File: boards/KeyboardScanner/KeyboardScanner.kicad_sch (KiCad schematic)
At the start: 20 parts, among them J1 Keyboard1, J2 Keyboard1, J3 Encoder, J4 Select, U5 ULN2803A, U8 4069

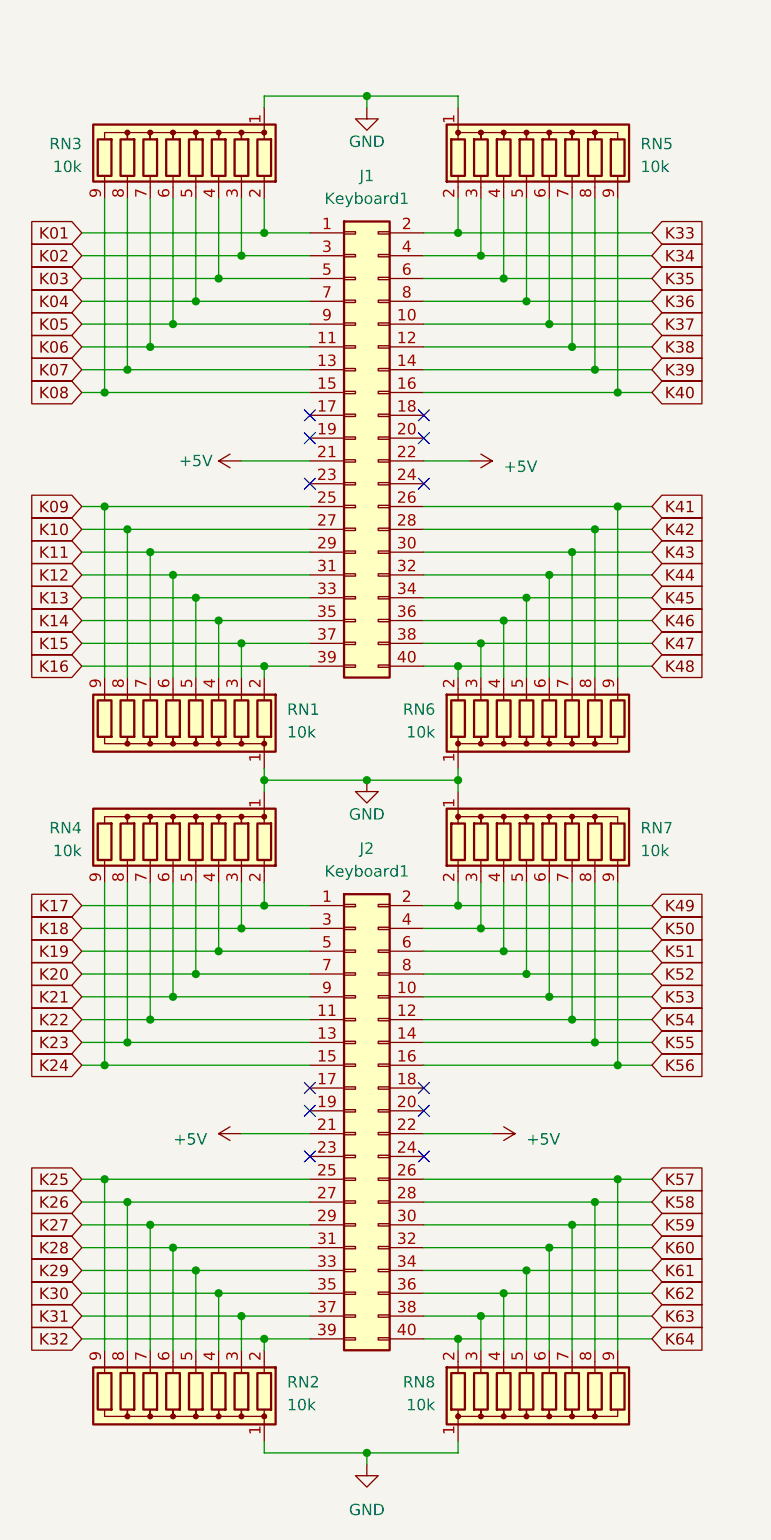
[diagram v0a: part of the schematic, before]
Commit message: Fixed KeyboardScanner schematics to fix open collector enable output
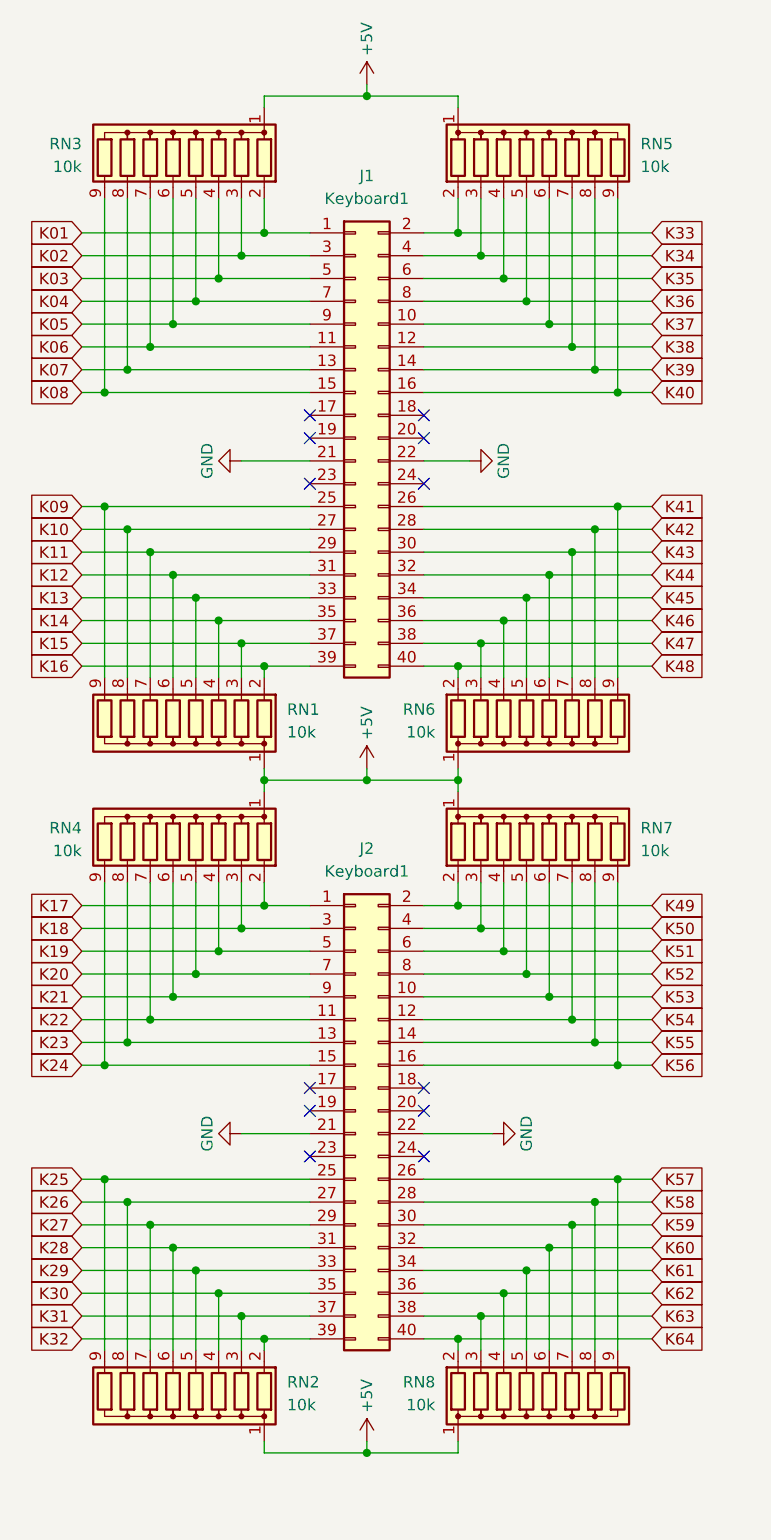
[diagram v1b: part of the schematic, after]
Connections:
- net +5V: now also RN1.1 (common), RN2.1 (common), RN3.1 (common), RN4.1 (common), RN5.1 (common), RN6.1 (common), RN7.1 (common), RN8.1 (common); no longer J1.21 (Pin_21), J1.22 (Pin_22), J2.21 (Pin_21), J2.22 (Pin_22)
- net GND: now also J1.21 (Pin_21), J1.22 (Pin_22), J2.21 (Pin_21), J2.22 (Pin_22); no longer RN1.1 (common), RN2.1 (common), RN3.1 (common), RN4.1 (common), RN5.1 (common), RN6.1 (common), RN7.1 (common), RN8.1 (common)

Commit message: Revert "Fixed KeyboardScanner schematics to fix open collector enable output"
This reverts commit 57decbb2314c6d76a4ad6cd92ca682e4977913ef.
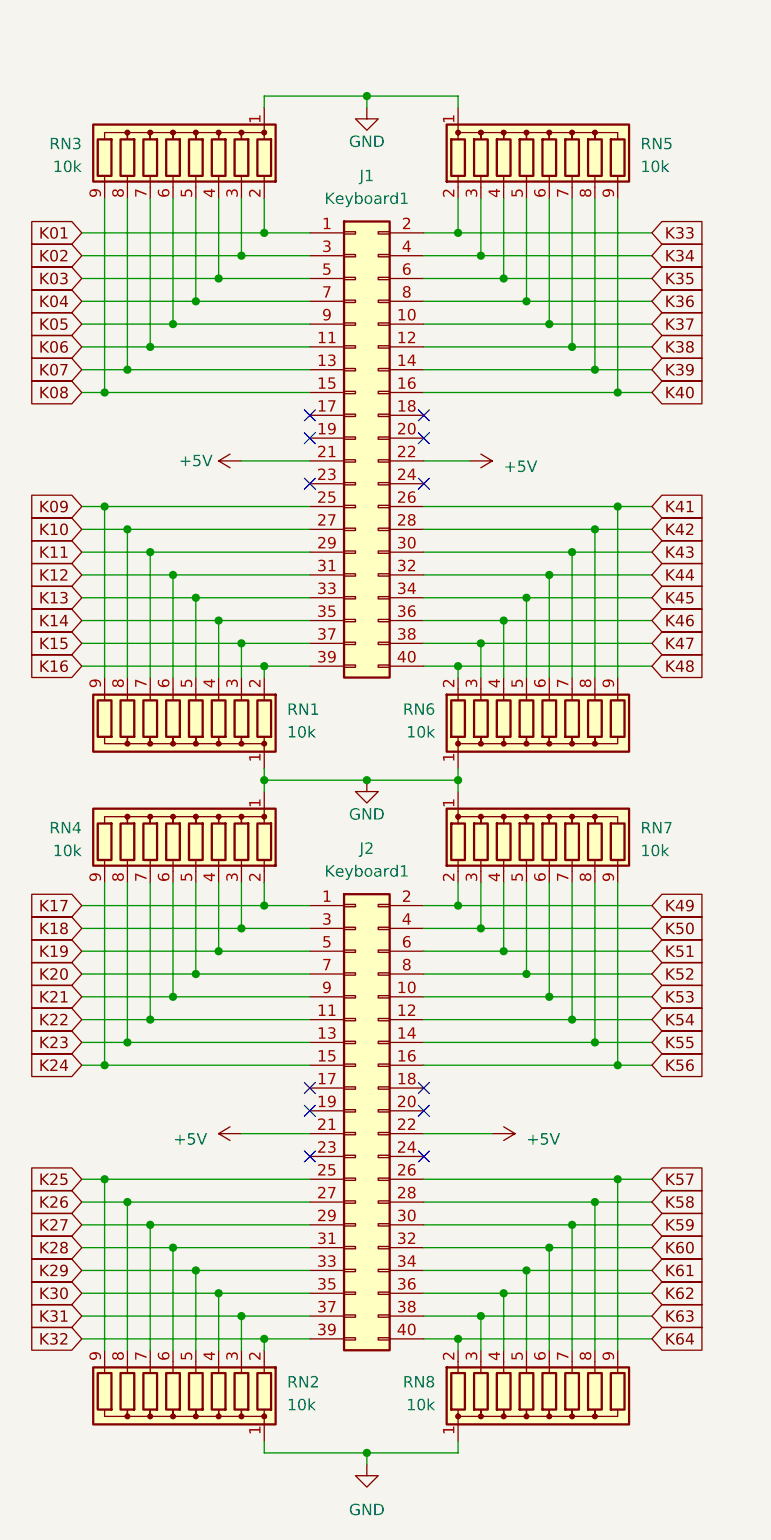
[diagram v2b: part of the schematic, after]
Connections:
- net +5V: now also J1.21 (Pin_21), J1.22 (Pin_22), J2.21 (Pin_21), J2.22 (Pin_22); no longer RN1.1 (common), RN2.1 (common), RN3.1 (common), RN4.1 (common), RN5.1 (common), RN6.1 (common), RN7.1 (common), RN8.1 (common)
- net GND: now also RN1.1 (common), RN2.1 (common), RN3.1 (common), RN4.1 (common), RN5.1 (common), RN6.1 (common), RN7.1 (common), RN8.1 (common); no longer J1.21 (Pin_21), J1.22 (Pin_22), J2.21 (Pin_21), J2.22 (Pin_22)

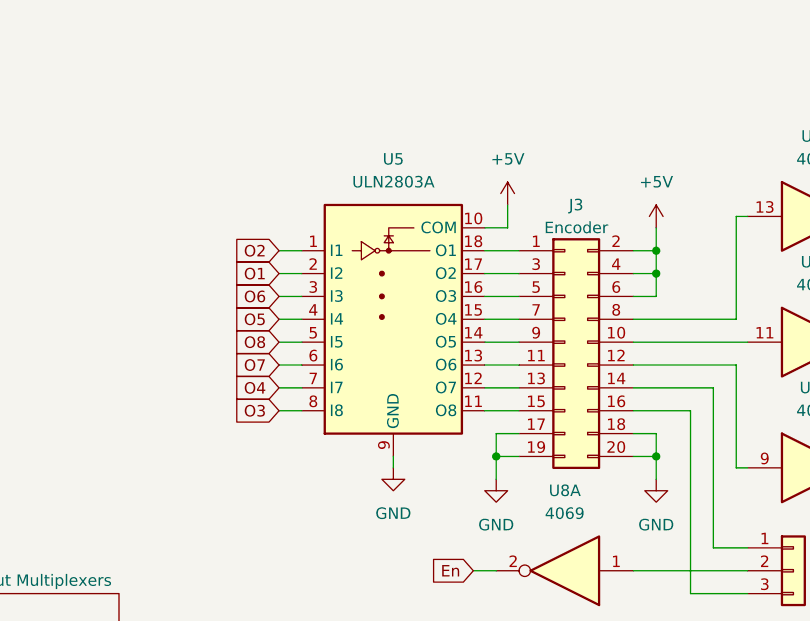
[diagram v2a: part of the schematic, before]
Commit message: Replaced inverting with non-inverting output buffer in KeyboardScanner to fix disabled open collector output
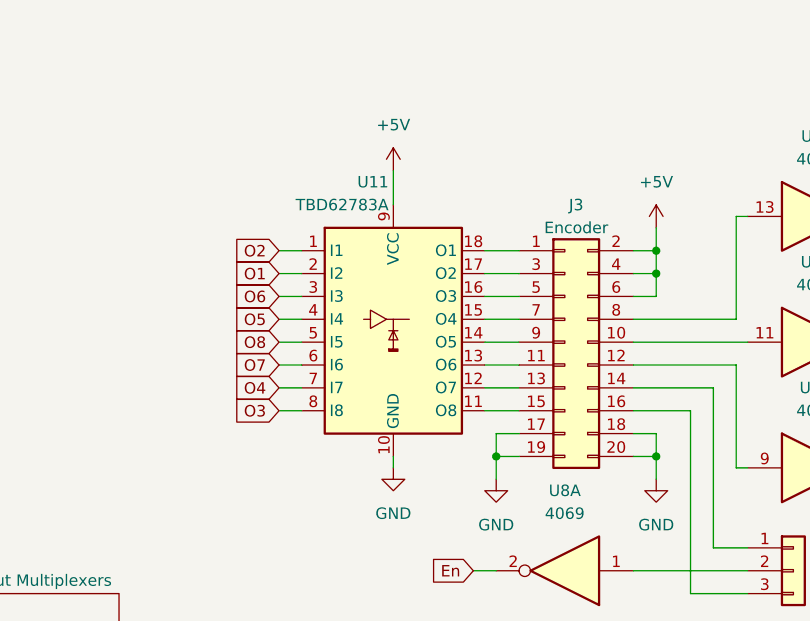
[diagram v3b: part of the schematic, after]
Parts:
- removed U5: ULN2803A, Package_DIP:DIP-18_W7.62mm, symbol Transistor_Array:ULN2803A
- added U11: TBD62783A, Package_DIP:DIP-18_W7.62mm, symbol Transistor_Array:TBD62783A
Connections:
- net +5V: now also U11.9 (VCC)
- net GND: now also U11.10 (GND)
- net O1: now also U11.2 (I2)
- net O2: now also U11.1 (I1)
- net O3: now also U11.8 (I8)
- net O4: now also U11.7 (I7)
- net O5: now also U11.4 (I4)
- net O6: now also U11.3 (I3)
- net O7: now also U11.6 (I6)
- net O8: now also U11.5 (I5)
- net at J3.1 (Pin_1): now also U11.18 (O1)
- net at J3.11 (Pin_11): now also U11.13 (O6)
- net at J3.13 (Pin_13): now also U11.12 (O7)
- net at J3.15 (Pin_15): now also U11.11 (O8)
- net at J3.3 (Pin_3): now also U11.17 (O2)
- net at J3.5 (Pin_5): now also U11.16 (O3)
- net at J3.7 (Pin_7): now also U11.15 (O4)
- net at J3.9 (Pin_9): now also U11.14 (O5)
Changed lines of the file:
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@@
 	(wire
 		(pts
-			(xy 194.31 48.26) (xy 191.77 48.26)
-		)
-		(stroke
-			(width 0)
-			(type default)
-		)
-	)
-	(wire
-		(pts
 			(xy 208.28 86.36) (xy 220.98 86.36)
 		)
@@
 	(wire
 		(pts
-			(xy 194.31 45.72) (xy 194.31 48.26)
-		)
-		(stroke
-			(width 0)
-			(type default)
-		)
-	)
-	(wire
-		(pts
 			(xy 58.42 90.17) (xy 58.42 88.9)
 		)
@@
 	(wire
 		(pts
+			(xy 181.61 41.91) (xy 181.61 45.72)
+		)
+		(stroke
+			(width 0)
+			(type default)
+		)
+	)
+	(wire
+		(pts
 			(xy 45.72 76.2) (xy 63.5 76.2)
 		)
@@
 	(symbol
 		(lib_id "power:+5V")
-		(at 194.31 45.72 0)
+		(at 181.61 41.91 0)
 		(unit 1)
 		(exclude_from_sim no)
@@
 		(fields_autoplaced yes)
 		(property "Reference" "#PWR010"
-			(at 194.31 49.53 0)
+			(at 181.61 45.72 0)
 			(effects
 				(font
@@
 		)
 		(property "Value" "+5V"
-			(at 194.31 40.64 0)
+			(at 181.61 36.83 0)
 			(effects
 				(font
@@
 		)
 		(property "Footprint" ""
-			(at 194.31 45.72 0)
+			(at 181.61 41.91 0)
 			(effects
 				(font
@@
 		)
 		(property "Datasheet" ""
-			(at 194.31 45.72 0)
+			(at 181.61 41.91 0)
 			(effects
 				(font
@@
 		)
 		(property "Description" "Power symbol creates a global label with name \"+5V\""
-			(at 194.31 45.72 0)
+			(at 181.61 41.91 0)
 			(effects
 				(font
@@
 	)
 	(symbol
-		(lib_id "Device:C_Polarized")
-		(at 194.31 125.73 0)
+		(lib_id "Transistor_Array:TBD62783A")
+		(at 181.61 58.42 0)
 		(unit 1)
 		(exclude_from_sim no)
@@
 		(on_board yes)
 		(dnp no)
-		(fields_autoplaced yes)
-		(property "Reference" "C10"
-			(at 198.12 123.5709 0)
+		(property "Reference" "U11"
+			(at 181.0894 43.18 0)
 			(effects
 				(font
 					(size 1.27 1.27)
 				)
-				(justify left)
+				(justify right)
 			)
 		)
-		(property "Value" "47uF"
-			(at 198.12 126.1109 0)
+		(property "Value" "TBD62783A"
+			(at 181.0894 45.72 0)
 			(effects
 				(font
 					(size 1.27 1.27)
 				)
-				(justify left)
+				(justify right)
 			)
 		)
-		(property "Footprint" "Capacitor_THT:CP_Radial_D6.3mm_P2.50mm"
-			(at 195.2752 129.54 0)
+		(property "Footprint" "Package_DIP:DIP-18_W7.62mm"
+			(at 181.61 72.39 0)
 			(effects
 				(font
@@
 			)
 		)
-		(property "Datasheet" "~"
-			(at 194.31 125.73 0)
+		(property "Datasheet" "http://toshiba.semicon-storage.com/info/docget.jsp?did=30523&prodName=TBD62783APG"
+			(at 173.99 48.26 0)
 			(effects
 				(font
@@
 			)
 		)
-		(property "Description" "Polarized capacitor"
-			(at 194.31 125.73 0)
+		(property "Description" "8-Channel Source Type Transistor Array, TTL and CMOS compatible, 500mA, 50V, DIP-18/SOP-18/SSOP-18/SOIC-18W"
+			(at 181.61 58.42 0)
 			(effects
 				(font
@@
 			)
 		)
+		(pin "1"
+		)
+		(pin "10"
+		)
+		(pin "11"
+		)
+		(pin "12"
+		)
+		(pin "13"
+		)
+		(pin "14"
+		)
+		(pin "15"
+		)
+		(pin "16"
+		)
+		(pin "17"
+		)
+		(pin "18"
+		)
 		(pin "2"
 		)
-		(pin "1"
+		(pin "3"
+		)
+		(pin "4"
+		)
+		(pin "5"
+		)
+		(pin "6"
+		)
+		(pin "7"
+		)
+		(pin "8"
+		)
+		(pin "9"
 		)
 		(instances
 			(project "KeyboardScanner"
 				(path "/cbea9b23-a5d5-4e12-8904-2e66ea6ed837"
-					(reference "C10")
+					(reference "U11")
 					(unit 1)
 				)
@@
 	)
 	(symbol
-		(lib_id "4xxx:4069")
-		(at 200.66 86.36 180)
+		(lib_id "Device:C_Polarized")
+		(at 194.31 125.73 0)
 		(unit 1)
 		(exclude_from_sim no)
@@
 		(dnp no)
 		(fields_autoplaced yes)
-		(property "Reference" "U8"
-			(at 200.66 77.47 0)
+		(property "Reference" "C10"
+			(at 198.12 123.5709 0)
 			(effects
 				(font
 					(size 1.27 1.27)
 				)
+				(justify left)
 			)
 		)
-		(property "Value" "4069"
-			(at 200.66 80.01 0)
+		(property "Value" "47uF"
+			(at 198.12 126.1109 0)
 			(effects
 				(font
 					(size 1.27 1.27)
 				)
+				(justify left)
 			)
 		)
-		(property "Footprint" "Package_DIP:DIP-14_W7.62mm"
-			(at 200.66 86.36 0)
+		(property "Footprint" "Capacitor_THT:CP_Radial_D6.3mm_P2.50mm"
+			(at 195.2752 129.54 0)
 			(effects
 				(font
@@
 			)
 		)
-		(property "Datasheet" "http://www.intersil.com/content/dam/Intersil/documents/cd40/cd4069ubms.pdf"
-			(at 200.66 86.36 0)
+		(property "Datasheet" "~"
+			(at 194.31 125.73 0)
 			(effects
 				(font
@@
 			)
 		)
-		(property "Description" "Hex inverter"
-			(at 200.66 86.36 0)
+		(property "Description" "Polarized capacitor"
+			(at 194.31 125.73 0)
 			(effects
 				(font
@@
 			)
 		)
-		(pin "1"
-		)
 		(pin "2"
 		)
-		(pin "3"
-		)
-		(pin "4"
-		)
-		(pin "5"
-		)
-		(pin "6"
-		)
-		(pin "8"
-		)
-		(pin "9"
-		)
-		(pin "10"
-		)
-		(pin "11"
-		)
-		(pin "12"
-		)
-		(pin "13"
-		)
-		(pin "14"
-		)
-		(pin "7"
+		(pin "1"
 		)
 		(instances
 			(project "KeyboardScanner"
 				(path "/cbea9b23-a5d5-4e12-8904-2e66ea6ed837"
-					(reference "U8")
+					(reference "C10")
 					(unit 1)
 				)
@@
 	)
 	(symbol
-		(lib_id "Transistor_Array:ULN2803A")
-		(at 181.61 55.88 0)
+		(lib_id "4xxx:4069")
+		(at 200.66 86.36 180)
 		(unit 1)
 		(exclude_from_sim no)
@@
 		(dnp no)
 		(fields_autoplaced yes)
-		(property "Reference" "U5"
-			(at 181.61 40.64 0)
+		(property "Reference" "U8"
+			(at 200.66 77.47 0)
 			(effects
 				(font
@@
 			)
 		)
-		(property "Value" "ULN2803A"
-			(at 181.61 43.18 0)
+		(property "Value" "4069"
+			(at 200.66 80.01 0)
 			(effects
 				(font
@@
 			)
 		)
-		(property "Footprint" "Package_DIP:DIP-18_W7.62mm"
-			(at 182.88 72.39 0)
+		(property "Footprint" "Package_DIP:DIP-14_W7.62mm"
+			(at 200.66 86.36 0)
 			(effects
 				(font
 					(size 1.27 1.27)
 				)
-				(justify left)
 				(hide yes)
 			)
 		)
-		(property "Datasheet" "http://www.ti.com/lit/ds/symlink/uln2803a.pdf"
-			(at 184.15 60.96 0)
+		(property "Datasheet" "http://www.intersil.com/content/dam/Intersil/documents/cd40/cd4069ubms.pdf"
+			(at 200.66 86.36 0)
 			(effects
 				(font
@@
 			)
 		)
-		(property "Description" "Darlington Transistor Arrays, SOIC18/DIP18"
-			(at 181.61 55.88 0)
+		(property "Description" "Hex inverter"
+			(at 200.66 86.36 0)
 			(effects
 				(font
@@
 		(pin "1"
 		)
-		(pin "10"
-		)
-		(pin "11"
-		)
-		(pin "12"
-		)
-		(pin "13"
-		)
-		(pin "14"
-		)
-		(pin "15"
-		)
-		(pin "16"
-		)
-		(pin "17"
-		)
-		(pin "18"
-		)
 		(pin "2"
 		)
@@
 		(pin "6"
 		)
-		(pin "7"
-		)
 		(pin "8"
 		)
 		(pin "9"
 		)
+		(pin "10"
+		)
+		(pin "11"
+		)
+		(pin "12"
+		)
+		(pin "13"
+		)
+		(pin "14"
+		)
+		(pin "7"
+		)
 		(instances
 			(project "KeyboardScanner"
 				(path "/cbea9b23-a5d5-4e12-8904-2e66ea6ed837"
-					(reference "U5")
+					(reference "U8")
 					(unit 1)
 				)
